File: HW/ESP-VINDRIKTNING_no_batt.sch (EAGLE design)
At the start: 47 parts, among them IC1 PI4ULS5V202UEX, IC3 CH340C, J1 USB-C_DONLY918-418K2022Y40000, Q1 MMDT3904, Q6 DMG2305UX, U1 ESP-12S

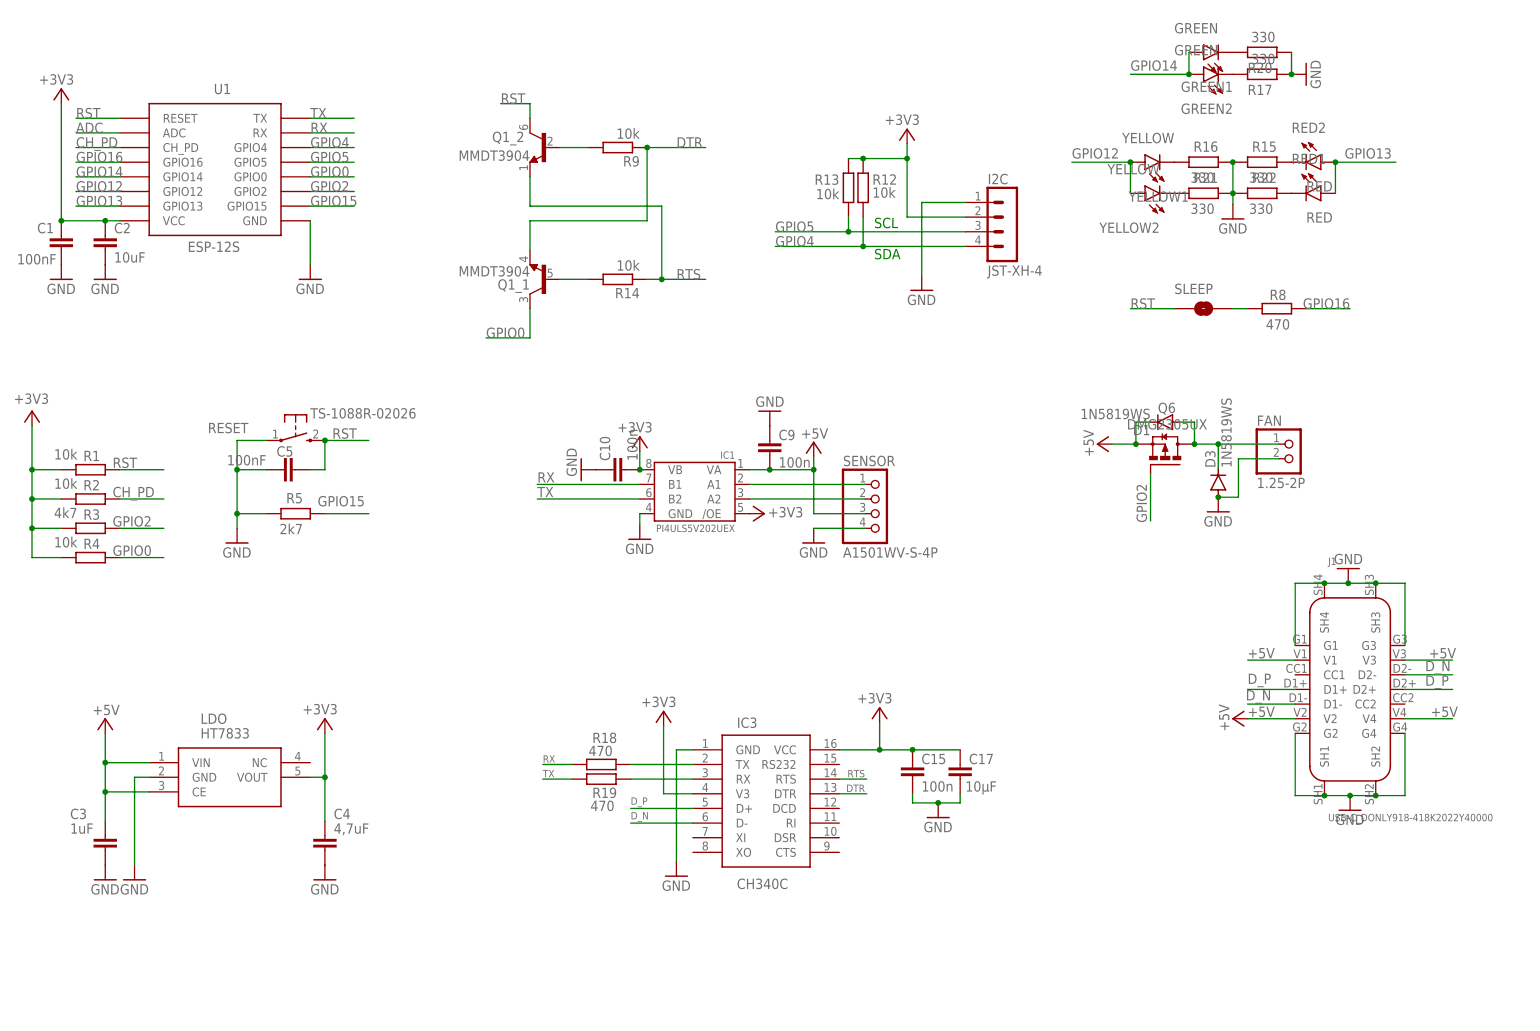
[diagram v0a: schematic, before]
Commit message: new
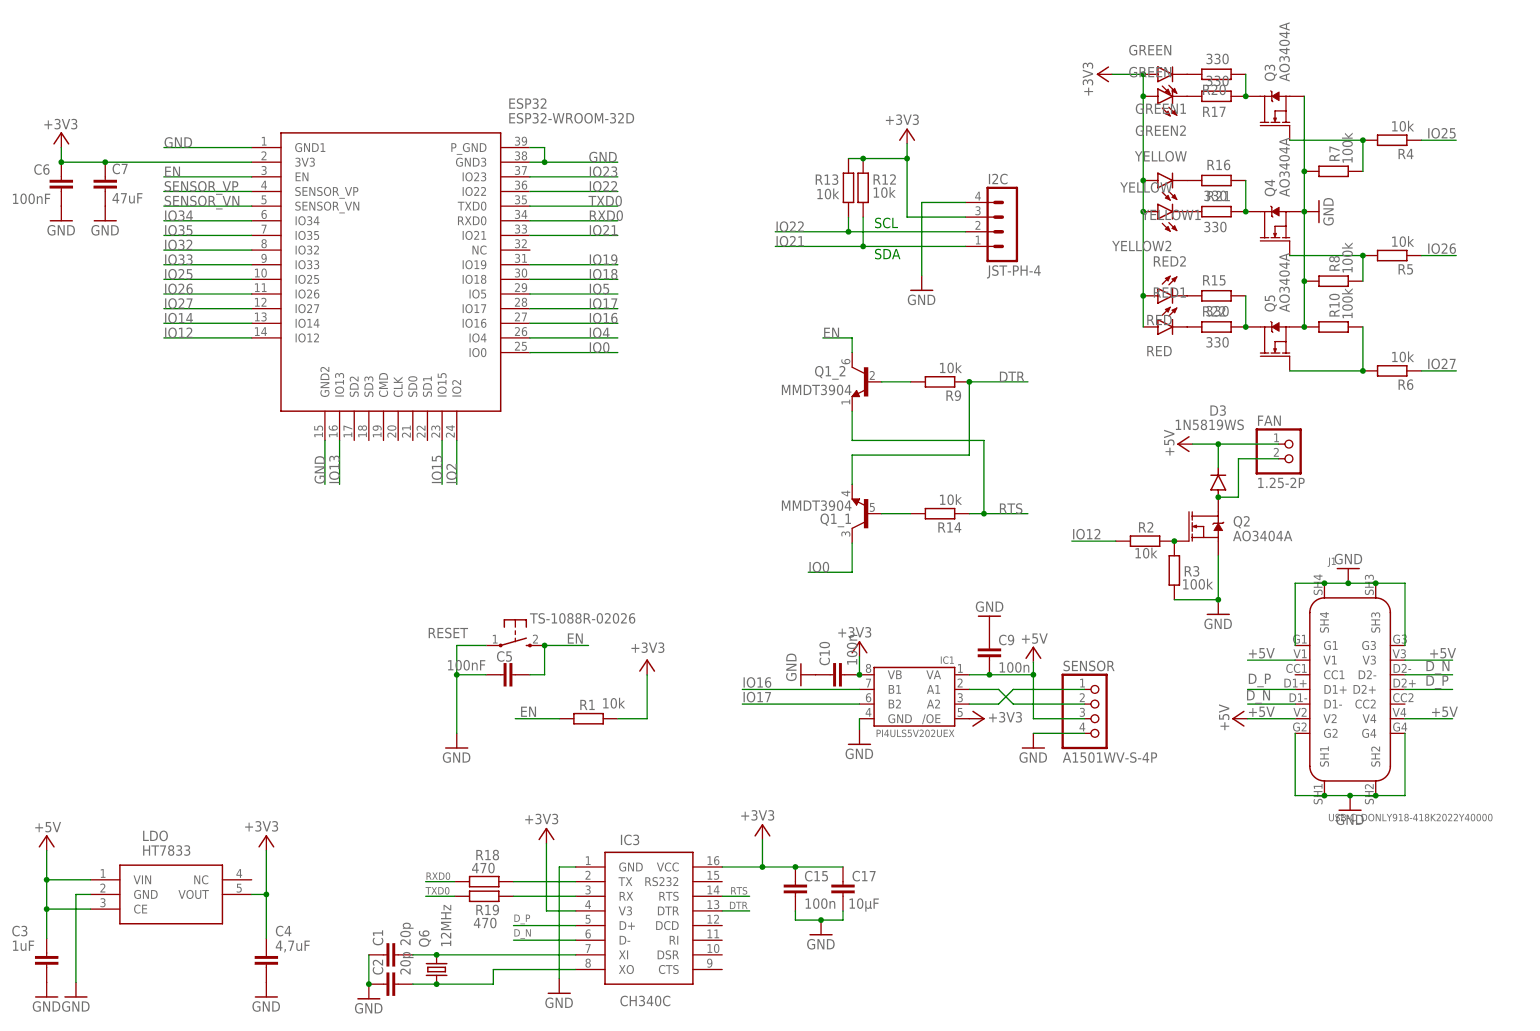
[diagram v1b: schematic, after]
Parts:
- removed D1: 1N5819WS, diode:DIODE-SOD323-R
- removed SLEEP: JUMPER-SMT_2_NO_NO-SILK, LasKKit-Connectors:JUMPER-SMT_2_NO_NO-SILK
- removed U1: ESP-12S, LasKKit-Modules:WIFI_ESP12SMD
- added C6: 100nF, rcl:C-EUC0603
- added C7: 47uF, rcl:C-EUC0603
- added ESP32: ESP32-WROOM-32D, LasKKit-Modules:ESP32-WROOM-32D
- added Q2, Q3, Q4, Q5: AO3404A, SparkFun-DiscreteSemi:MOSFET-NCH-AO3404A
- added R10, R7: 100k, rcl:R-EU_R0402
- added R6: 10k, rcl:R-EU_R0402
- C1: value 100nF -> 20p; device rcl:C-EUC0603 -> rcl:C-EUC0402
- C2: value 10uF -> 20p; device rcl:C-EUC0603 -> rcl:C-EUC0402
- I2C: value JST-XH-4 -> JST-PH-4; device LasKKit-Connectors:JST-XH-4 -> LasKKit-Connectors:JST-PH-4; LCSC_PART (none) -> C2321
- Q6: value DMG2305UX -> 12MHz; device transistor-power:FDN360P -> crystal-geyer_V1_0:KX-7; LCSC_PART C144153 -> C97242
- R3: value 4k7 -> 100k
- R5: value 2k7 -> 10k
- R8: value 470 -> 100k
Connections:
- removed net ADC: U1.ADC
- removed net CH_PD: R2.2, U1.CH_PD
- removed net GPIO0: Q1_1.C, R4.2, U1.GPIO0
- removed net GPIO12: U1.GPIO12, YELLOW1.A, YELLOW2.A
- removed net GPIO13: RED1.A, RED2.A, U1.GPIO13
- removed net GPIO14: GREEN1.A, GREEN2.A, U1.GPIO14
- removed net GPIO15: R5.1, U1.GPIO15
- removed net GPIO16: R8.2, U1.GPIO16
- removed net GPIO2: Q6.G, R3.2, U1.GPIO2
- removed net GPIO4: I2C.4, R12.1, U1.GPIO4
- removed net GPIO5: I2C.3, R13.1, U1.GPIO5
- removed net RST: C5.2, Q1_2.C, R1.2, RESET.3, SLEEP.1, U1.RESET
- removed net RX: IC1.B1, R18.1, U1.RX
- removed net TX: IC1.B2, R19.1, U1.TX
- new net EN: C5.2, ESP32.EN, Q1_2.C, R1.2, RESET.3
- new net IO0: ESP32.IO0, Q1_1.C
- new net IO12: ESP32.IO12, R2.2
- new net IO13: ESP32.IO13
- new net IO14: ESP32.IO14
- new net IO15: ESP32.IO15
- new net IO16: ESP32.IO16, IC1.B1
- new net IO17: ESP32.IO17, IC1.B2
- new net IO18: ESP32.IO18
- new net IO19: ESP32.IO19
- new net IO2: ESP32.IO2
- new net IO21: ESP32.IO21, I2C.4, R12.1
- new net IO22: ESP32.IO22, I2C.3, R13.1
- new net IO23: ESP32.IO23
- new net IO25: ESP32.IO25, R4.1
- new net IO26: ESP32.IO26, R5.1
- new net IO27: ESP32.IO27, R6.1
- new net IO32: ESP32.IO32
- new net IO33: ESP32.IO33
- new net IO34: ESP32.IO34
- new net IO35: ESP32.IO35
- new net IO4: ESP32.IO4
- new net IO5: ESP32.IO5
- new net N$10: Q4.G, R5.2, R8.2
- new net N$17: Q3.G, R4.2, R7.2
- new net N$2: D3.A, FAN.2, Q2.D
- new net N$3: Q2.G, R2.1, R3.1
- new net N$4: C1.2, IC3.XI, Q6.2
- new net N$5: Q5.D, R15.2, R22.2
- new net N$7: Q3.D, R17.2, R20.2
- new net N$9: Q5.G, R10.2, R6.2
- new net RXD0: ESP32.RXD0, R18.1
- new net SENSOR_VN: ESP32.SENSOR_VN
- new net SENSOR_VP: ESP32.SENSOR_VP
- new net TXD0: ESP32.TXD0, R19.1
- net +3V3: now also C6.1, C7.1, ESP32.3V3, GREEN1.A, GREEN2.A, RED1.A, RED2.A, YELLOW1.A, YELLOW2.A; no longer C1.1, C2.1, R2.1, R3.1, R4.1, U1.VCC
- net +5V: now also D3.C, FAN.1; no longer D1.C, Q6.S
- net GND: now also C1.1, C2.1, C6.2, C7.2, ESP32.GND1, ESP32.GND2, ESP32.GND3, ESP32.P_GND, Q2.S, Q3.S, Q4.S, Q5.S, R10.1, R3.2, R7.1, R8.1; no longer C1.2, C2.2, D3.A, FAN.2, R15.2, R16.1, R17.2, R20.2, R21.1, R22.2, R5.2, U1.GND
- net N$18: now also C2.2, IC3.XO, Q6.1; no longer D1.A, D3.C, FAN.1, Q6.D
- net N$6: now also Q4.D, R16.1, R21.1; no longer R8.1, SLEEP.2
- net RX_: now also SENSOR.2; no longer SENSOR.1
- net TX_: now also SENSOR.1; no longer SENSOR.2
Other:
- moved on the sheet: C1, C10, C15, C17, C2, C3, C4, C5, C9, GREEN1, GREEN2, IC1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
